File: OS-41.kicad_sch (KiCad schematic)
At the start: 65 parts, among them J1 Conn_02x03_Counter_Clockwise, J2 Conn_01x02_Pin, J3 Conn_01x02_Pin, J4 Conn_Coaxial, SW4 SW_Push, U1 BME280, U2 SI4432-B1-FMR, U3 MCP1640x-xCHY, U4 ATGM336H-5N31, U7 STM32F103C8Tx, Y1 32.768KHz 12.5pF, Y2 8MHz 12pF, Y3 30MHz 10pF

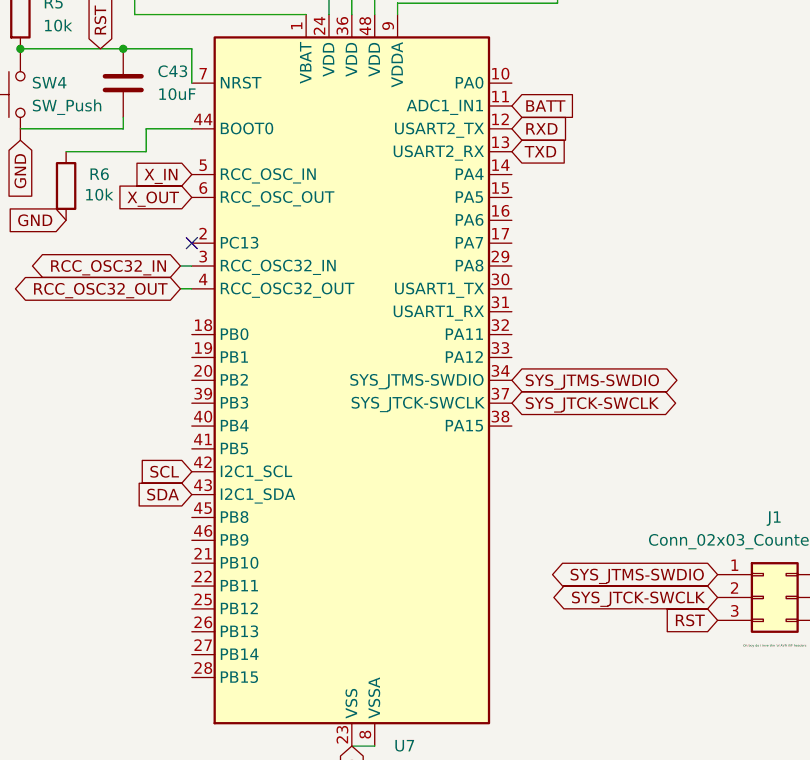
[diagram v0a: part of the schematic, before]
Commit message: Continue layout
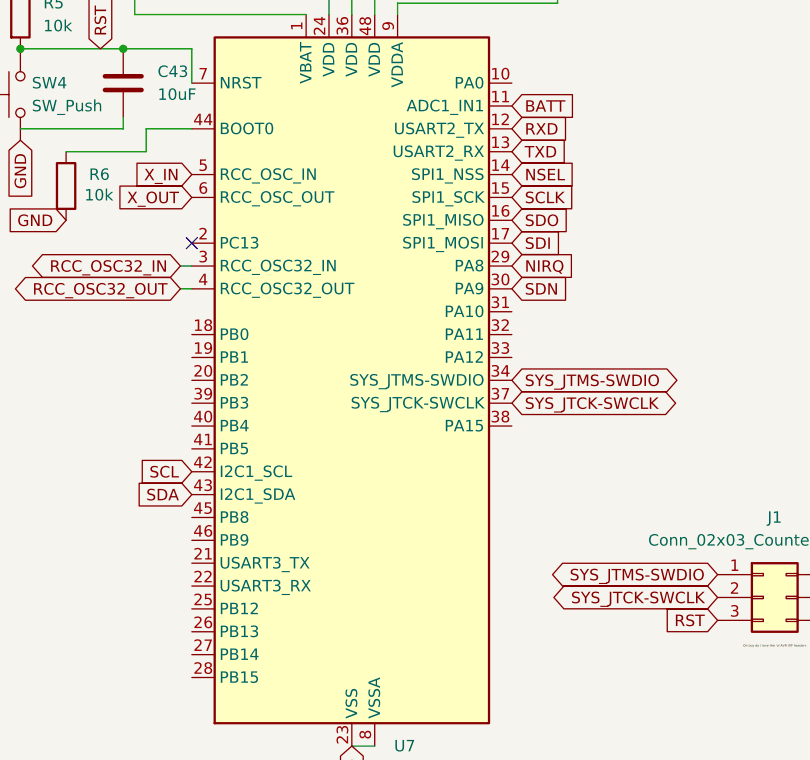
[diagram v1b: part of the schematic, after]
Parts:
- SW4: footprint Button_Switch_THT:SW_PUSH_6mm -> libsos41:SMD_SW_NEW_REDONE
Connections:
- net NIRQ: now also U7.29 (PA8)
- net NSEL: now also U7.14 (PA4)
- net SCLK: now also U7.15 (PA5)
- net SDI: now also U7.17 (PA7)
- net SDN: now also U7.30 (PA9)
- net SDO: now also U7.16 (PA6)
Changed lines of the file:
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@@
 		)
 	)
+	(global_label "NIRQ"
+		(shape input)
+		(at 326.39 76.2 0)
+		(effects
+			(font
+				(size 1.27 1.27)
+			)
+			(justify left)
+		)
+		(property "Intersheetrefs" "${INTERSHEET_REFS}"
+			(at 326.39 76.2 90)
+			(effects
+				(font
+					(size 1.27 1.27)
+				)
+				(hide yes)
+			)
+		)
+	)
+	(global_label "SDO"
+		(shape input)
+		(at 326.39 71.12 0)
+		(effects
+			(font
+				(size 1.27 1.27)
+			)
+			(justify left)
+		)
+		(property "Intersheetrefs" "${INTERSHEET_REFS}"
+			(at 326.39 71.12 0)
+			(effects
+				(font
+					(size 1.27 1.27)
+				)
+				(hide yes)
+			)
+		)
+	)
 	(global_label "VCC"
 		(shape input)
@@
 		)
 	)
+	(global_label "SDN"
+		(shape input)
+		(at 326.39 78.74 0)
+		(effects
+			(font
+				(size 1.27 1.27)
+			)
+			(justify left)
+		)
+		(property "Intersheetrefs" "${INTERSHEET_REFS}"
+			(at 326.39 78.74 90)
+			(effects
+				(font
+					(size 1.27 1.27)
+				)
+				(hide yes)
+			)
+		)
+	)
 	(global_label "RST"
 		(shape input)
@@
 		)
 	)
+	(global_label "SDI"
+		(shape input)
+		(at 326.39 73.66 0)
+		(effects
+			(font
+				(size 1.27 1.27)
+			)
+			(justify left)
+		)
+		(property "Intersheetrefs" "${INTERSHEET_REFS}"
+			(at 326.39 73.66 0)
+			(effects
+				(font
+					(size 1.27 1.27)
+				)
+				(hide yes)
+			)
+		)
+	)
 	(global_label "TXD"
 		(shape input)
@@
 		)
 	)
+	(global_label "SCLK"
+		(shape input)
+		(at 326.39 68.58 0)
+		(effects
+			(font
+				(size 1.27 1.27)
+			)
+			(justify left)
+		)
+		(property "Intersheetrefs" "${INTERSHEET_REFS}"
+			(at 326.39 68.58 0)
+			(effects
+				(font
+					(size 1.27 1.27)
+				)
+				(hide yes)
+			)
+		)
+	)
 	(global_label "GND"
 		(shape input)
@@
 		)
 	)
+	(global_label "NSEL"
+		(shape input)
+		(at 326.39 66.04 0)
+		(effects
+			(font
+				(size 1.27 1.27)
+			)
+			(justify left)
+		)
+		(property "Intersheetrefs" "${INTERSHEET_REFS}"
+			(at 326.39 66.04 90)
+			(effects
+				(font
+					(size 1.27 1.27)
+				)
+				(hide yes)
+			)
+		)
+	)
 	(global_label "GND"
 		(shape input)
@@
 			)
 		)
-		(property "Footprint" "Button_Switch_THT:SW_PUSH_6mm"
+		(property "Footprint" "libsos41:SMD_SW_NEW_REDONE"
 			(at 266.7 57.15 0)
 			(effects
@@
 		)
 		(pin "22"
+			(alternate "USART3_RX")
 		)
 		(pin "28"
@@
 		)
 		(pin "16"
+			(alternate "SPI1_MISO")
 		)
 		(pin "17"
+			(alternate "SPI1_MOSI")
 		)
 		(pin "32"
@@
 		)
 		(pin "15"
+			(alternate "SPI1_SCK")
 		)
 		(pin "13"
@@
 		)
 		(pin "31"
-			(alternate "USART1_RX")
 		)
 		(pin "26"
@@
 		)
 		(pin "30"
-			(alternate "USART1_TX")
 		)
 		(pin "48"
@@
 		)
 		(pin "14"
+			(alternate "SPI1_NSS")
 		)
 		(pin "21"
+			(alternate "USART3_TX")
 		)
 		(pin "23"
